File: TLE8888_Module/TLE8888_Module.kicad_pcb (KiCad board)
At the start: 4 copper layers, 100 x 22 mm, 41 parts, among them J1 Conn_01x01, J2 Conn_02x39_Odd_Even, Q1 IPD30N06S2L-23, U2 TLE8888QK

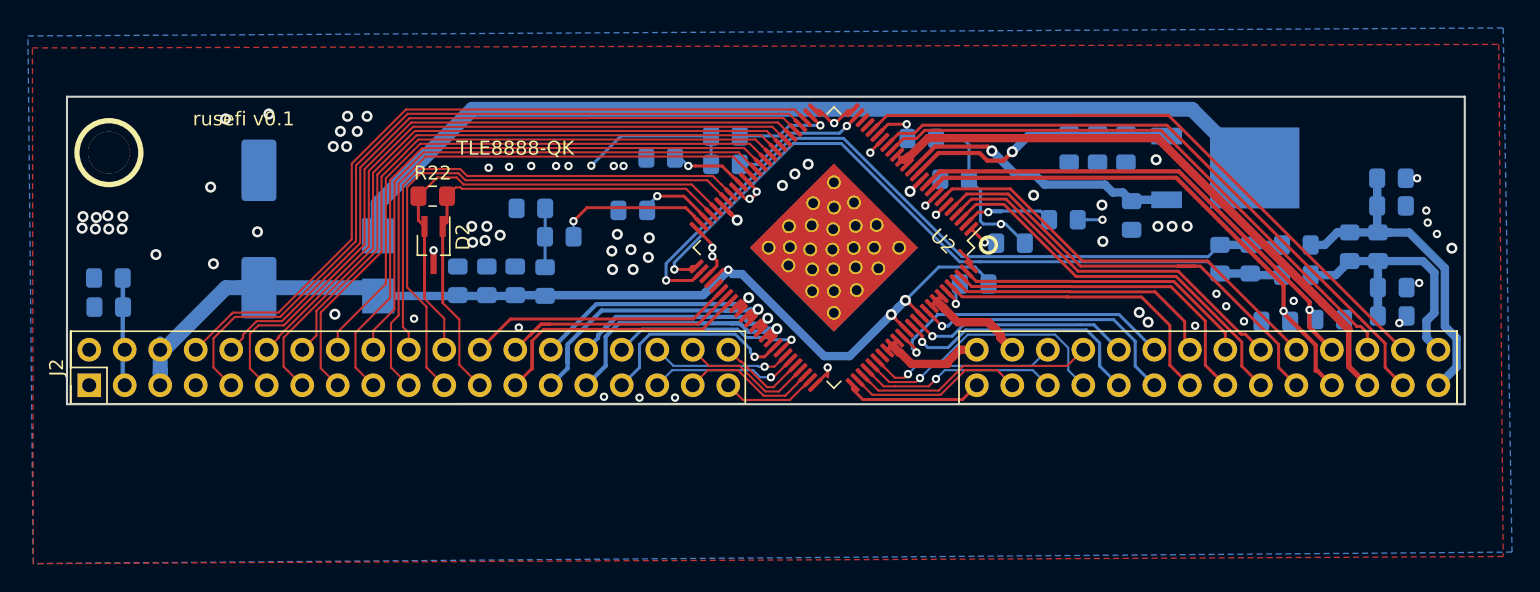
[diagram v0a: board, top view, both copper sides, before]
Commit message: sync
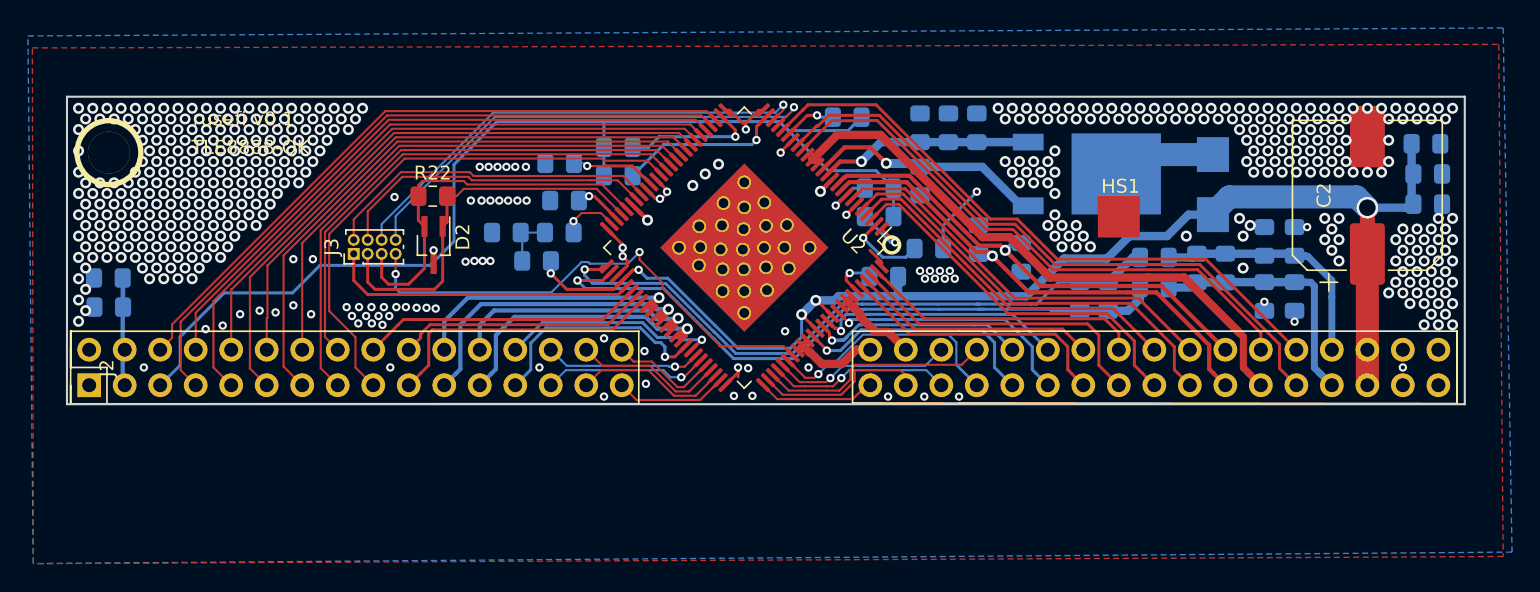
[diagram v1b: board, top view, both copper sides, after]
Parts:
- added HS1: Heatsink, Heatsink:HEATSINK, F.Cu at (95.4, 25.9)
- added HS2: Heatsink, Heatsink:HEATSINK, B.Cu at (68.8, 32.5)
- added J3: Conn_02x04_Odd_Even, Connector_PinHeader_1.00mm:PinHeader_2x04_P1.00mm_Vertical, F.Cu at (40.5, 31.2)
- C2: moved to F.Cu
- moved C2 79.3 mm to (113.0, 27.1)
- moved R21 69.6 mm to (117.3, 27.7), turned to 180 degrees
- moved C16 67.9 mm to (117.2, 23.4), turned to 0 degrees
- moved C1 65.7 mm to (117.3, 25.5), turned to 0 degrees
- moved D1 60.0 mm to (102.0, 26.3)
- moved C5 22.5 mm to (88.3, 31.5), turned to 270 degrees
- moved C4 22.0 mm to (85.2, 30.2), turned to 90 degrees
- moved C11 15.3 mm to (81.0, 26.0)
- moved R16 11.2 mm to (105.7, 34.3), turned to 90 degrees
- moved R15 11.0 mm to (100.8, 32.3), turned to 90 degrees
- moved C15 11.0 mm to (102.9, 32.3), turned to 90 degrees
- moved R17 10.9 mm to (107.8, 34.3), turned to 90 degrees
- moved C10 10.8 mm to (81.0, 22.2), turned to 90 degrees
- moved C8 10.8 mm to (85.1, 22.2), turned to 90 degrees
- moved C9 10.8 mm to (83.1, 22.2), turned to 90 degrees
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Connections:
- J2 pad 10: /INJ_IN_3 -> /IGN_IN_1
- J2 pad 11: /INJ_IN_4 -> /IGN_IN_2
- J2 pad 12: /IGN_IN_1 -> /IGN_IN_3
- J2 pad 13: /IGN_IN_2 -> /IGN_IN_4
- J2 pad 14: /IGN_IN_3 -> /IN_9
- J2 pad 15: /IGN_IN_4 -> /IN_10
- J2 pad 16: /IN_9 -> /IN_11
- J2 pad 17: /IN_10 -> /IN_12
- J2 pad 18: /IN_11 -> /OUT_18
- J2 pad 19: /IN_12 -> /OUT_16
- J2 pad 20: /CAN_RX -> /OUT_17
- J2 pad 21: /CAN_TX -> /OUT_2
- J2 pad 22: /CAN_H -> /OUT_1
- J2 pad 23: /CAN_L -> /OUT_4
- J2 pad 24: /OUT_18 -> /OUT_3
- J2 pad 25: /OUT_16 -> /OUT_15
- J2 pad 26: /OUT_17 -> /OUT_14
- J2 pad 27: /OUT_2 -> /DFB_9
- J2 pad 28: /OUT_1 -> /DFB_8
- J2 pad 29: /OUT_4 -> /DFB_10
- J2 pad 30: /OUT_3 -> /OUT_9
- J2 pad 31: /OUT_15 -> /OUT_10
- J2 pad 32: /OUT_14 -> /OUT_8
- J2 pad 33: /DFB_9 -> /DFB_11
- J2 pad 34: /DFB_8 -> /OUT_5
- J2 pad 35: /DFB_10 -> /OUT_11
- J2 pad 36: /OUT_9 -> /OUT_6
- J2 pad 37: /OUT_10 -> /OUT_12
- J2 pad 38: /OUT_8 -> /DFB_13
- J2 pad 39: /DFB_11 -> /OUT_13
- J2 pad 40: /OUT_5 -> /DFB_12
- J2 pad 41: /OUT_11 -> /OUT_24
- J2 pad 42: /OUT_6 -> /OUT_23
- J2 pad 43: /OUT_12 -> /OUT_21
- J2 pad 44: /DFB_13 -> /OUT_22
- J2 pad 45: /OUT_13 -> /IGN_OUT_1
- J2 pad 46: /DFB_12 -> /IGN_OUT_2
- J2 pad 47: /OUT_23 -> /IGN_OUT_3
- J2 pad 48: /OUT_22 -> /IGN_OUT_4
- J2 pad 49: /OUT_21 -> /CSN
- J2 pad 5: /12V -> /VDD
- J2 pad 50: /OUT_24 -> /SDO
- J2 pad 51: /IGN_OUT_1 -> /SIP
- J2 pad 52: /IGN_OUT_2 -> /FCLP
- J2 pad 53: /IGN_OUT_3 -> /5V1
- J2 pad 54: /IGN_OUT_4 -> /5V2
- J2 pad 55: /CSN -> /OUT_7
- J2 pad 56: /SDO -> /OUT_20
- J2 pad 57: /SIP -> /OUT_19
- J2 pad 58: /FCLP -> /CRNK_MCU
- J2 pad 59: /5V1 -> /CRNK+
- J2 pad 6: /12V -> /INJ_IN_1
- J2 pad 60: /5V2 -> /CRNK-
- J2 pad 61: /OUT_7 -> /12V
- J2 pad 62: /OUT_20 -> /12V
- J2 pad 63: /OUT_19 -> /V5V
- J2 pad 64: /CRNK_MCU -> /V5V
- J2 pad 65: /CRNK+ -> GND
- J2 pad 66: /CRNK- -> GND
- J2 pad 7: /VDD -> /INJ_IN_2
- J2 pad 8: /INJ_IN_1 -> /INJ_IN_3
- J2 pad 9: /INJ_IN_2 -> /INJ_IN_4
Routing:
- net Net-(D1-Pad1): track 69.6 -> 7.49 mm
- net /LIN_IO: track 0.00 -> 36.1 mm, vias 0 -> 2
- net /LIN_TX: track 0.00 -> 35.3 mm, vias 0 -> 1
- net /LIN_RX: track 0.00 -> 35.1 mm, vias 0 -> 1
- net /MAIN_RELAY: track 0.00 -> 22.4 mm
- net /CAN_TX: track 39.3 -> 23.0 mm
- net /VDD: track 94.6 -> 78.6 mm, vias 2 -> 0
- net /12V: track 81.8 -> 94.6 mm, vias 3 -> 5
- net /CAN_RX: track 36.8 -> 24.1 mm
- net Net-(C12-Pad1): track 56.5 -> 49.3 mm
- net /CAN_H: track 34.6 -> 27.4 mm
- net /KEY: track 11.2 -> 4.43 mm
- net /INJ_IN_2: track 56.0 -> 49.3 mm
- net /INJ_IN_1: track 54.2 -> 47.6 mm
- net /CRNK+: track 24.2 -> 17.8 mm
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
